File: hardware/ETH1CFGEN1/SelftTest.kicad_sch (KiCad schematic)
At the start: 28 parts, among them U801 TL074HIPWR, U802 TL074HIPWR, U803 TLA2528IRTER

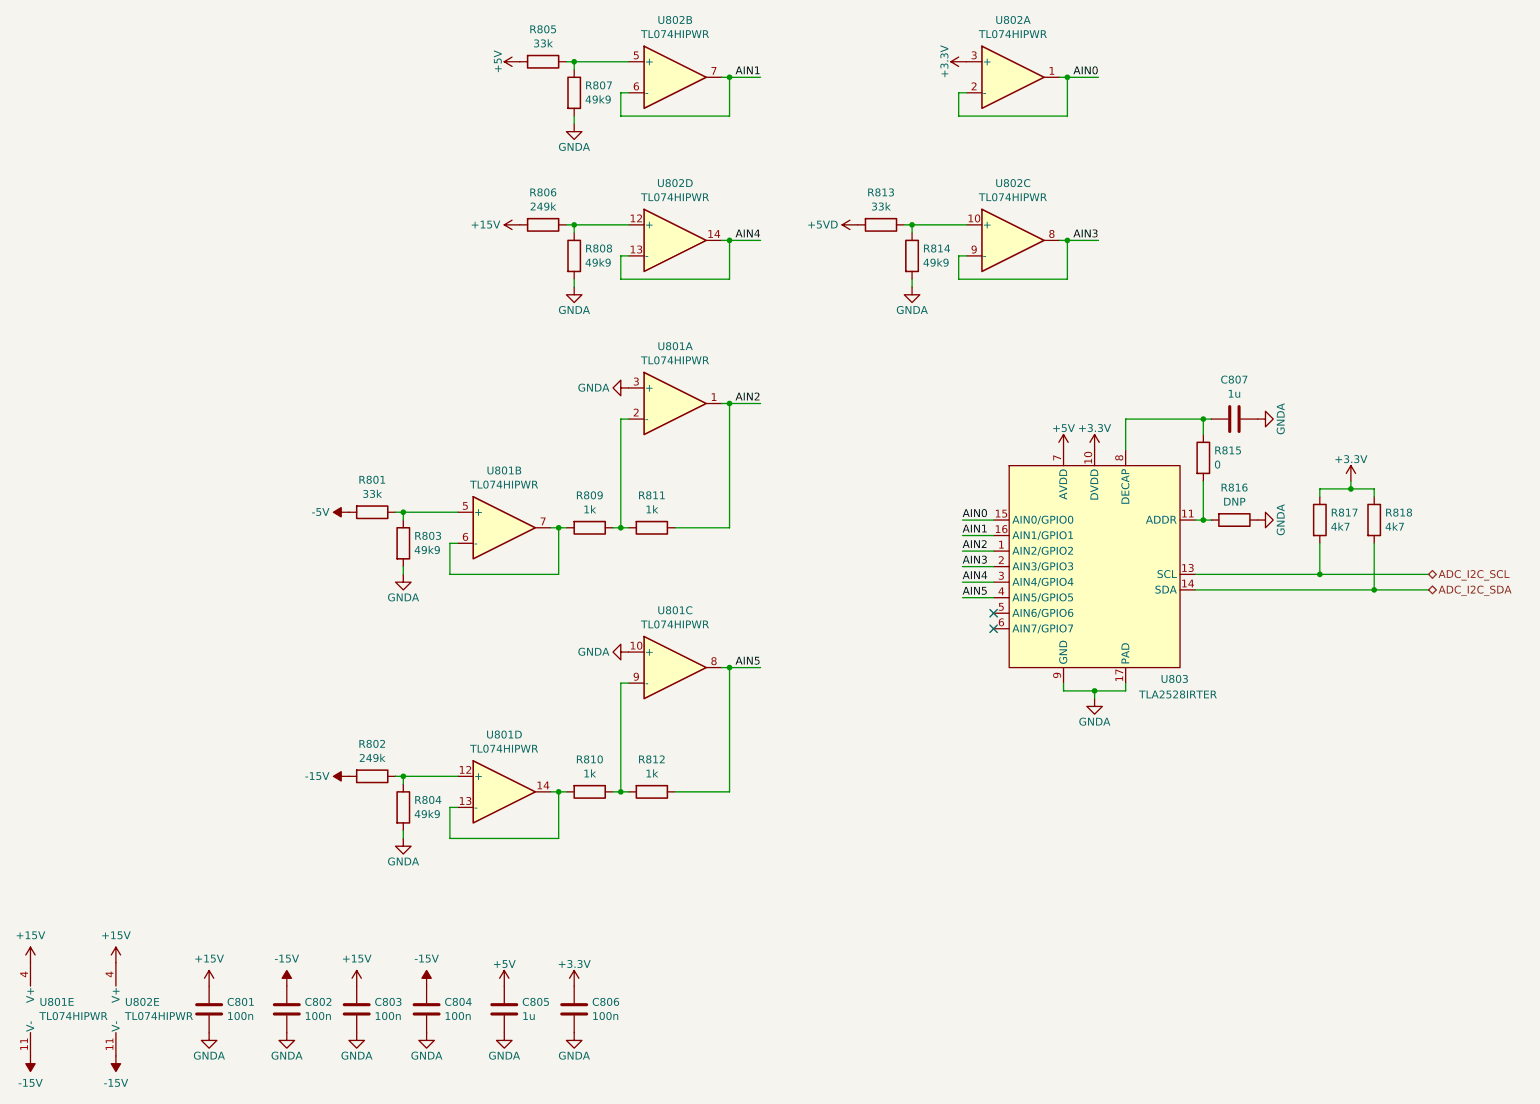
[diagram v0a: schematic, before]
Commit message: PCB design
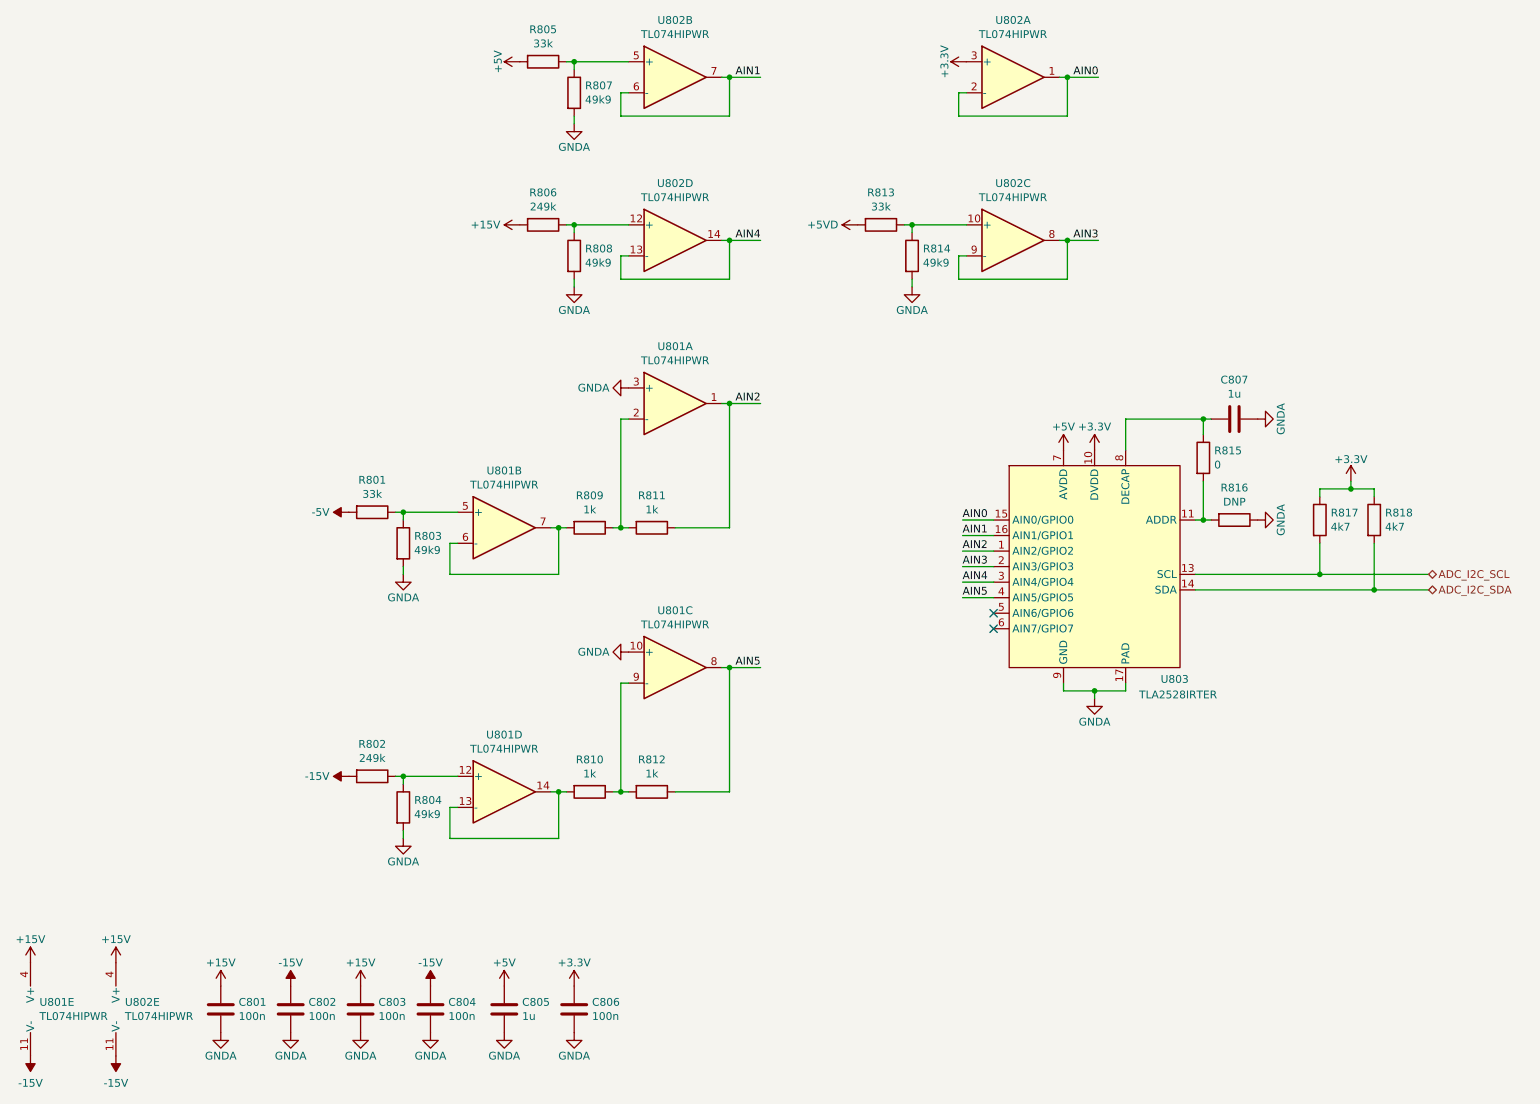
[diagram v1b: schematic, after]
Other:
- moved on the sheet: C801, C802, C803, C804
